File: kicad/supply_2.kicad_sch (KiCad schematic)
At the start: 24 parts, among them J2 +3.3, J3 GND, P1 USB_C_Plug_USB2.0, U3 TP4056-42-ESOP8, U4 USBLC6-2P6, U5 U8205A, U6 DW01A, U7 AMS1117-3.3, U8 Switch

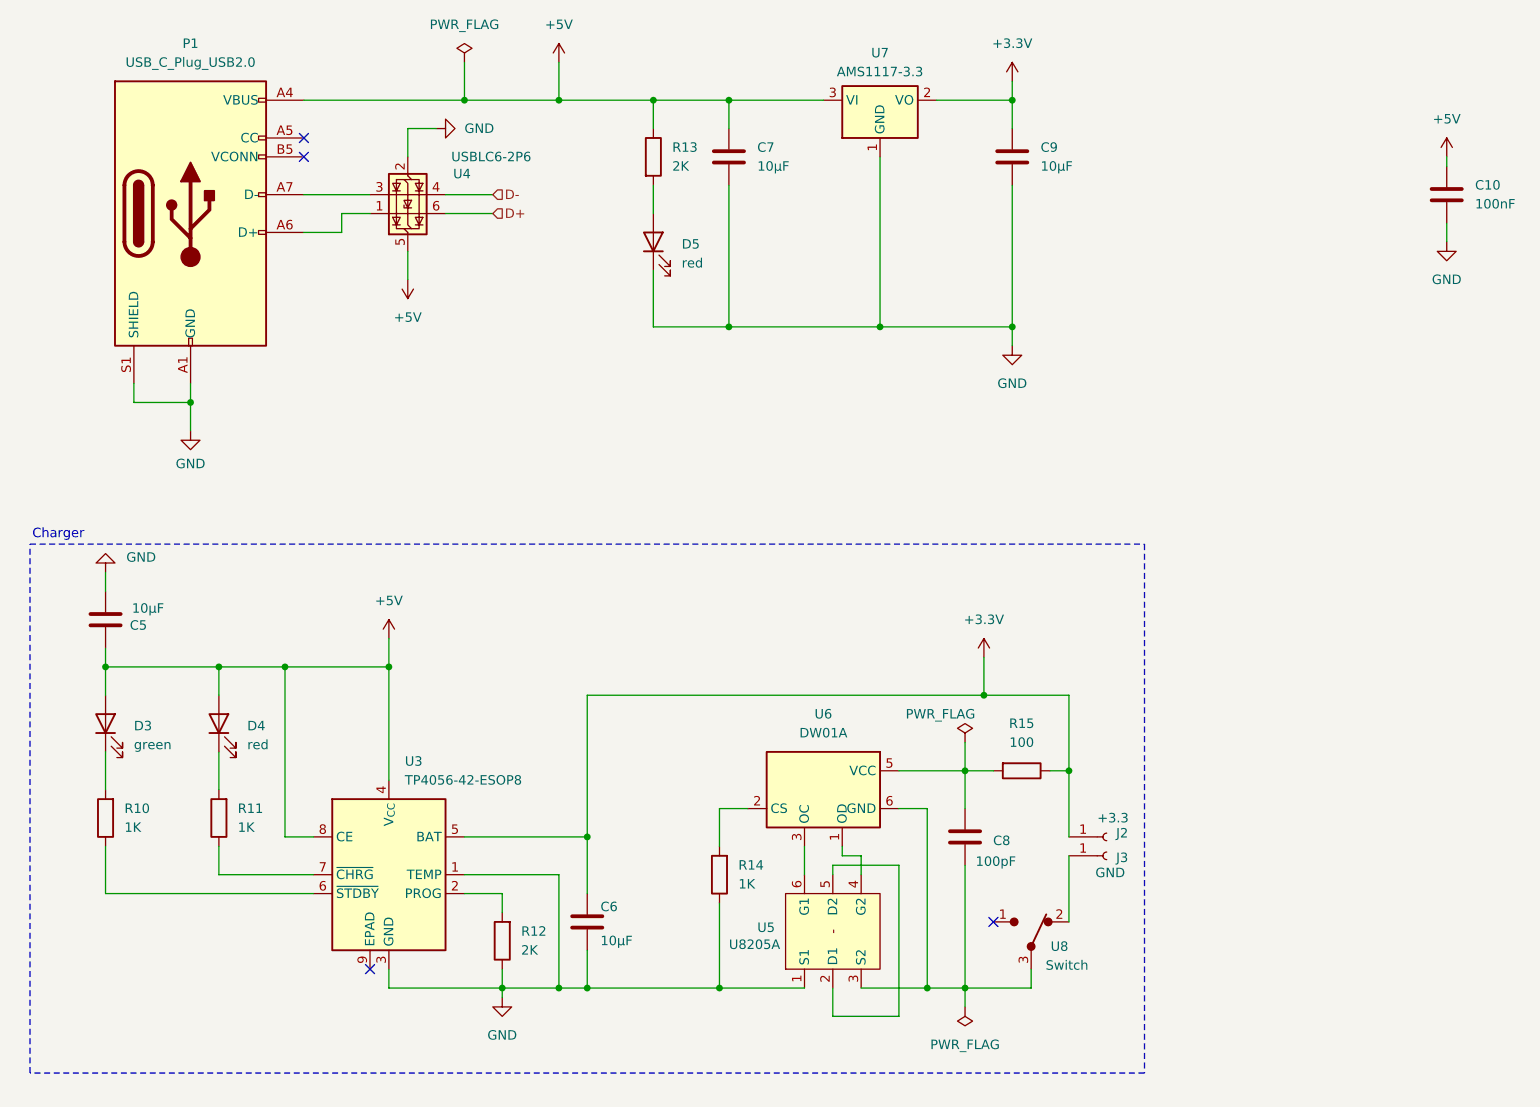
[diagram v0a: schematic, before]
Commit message: init
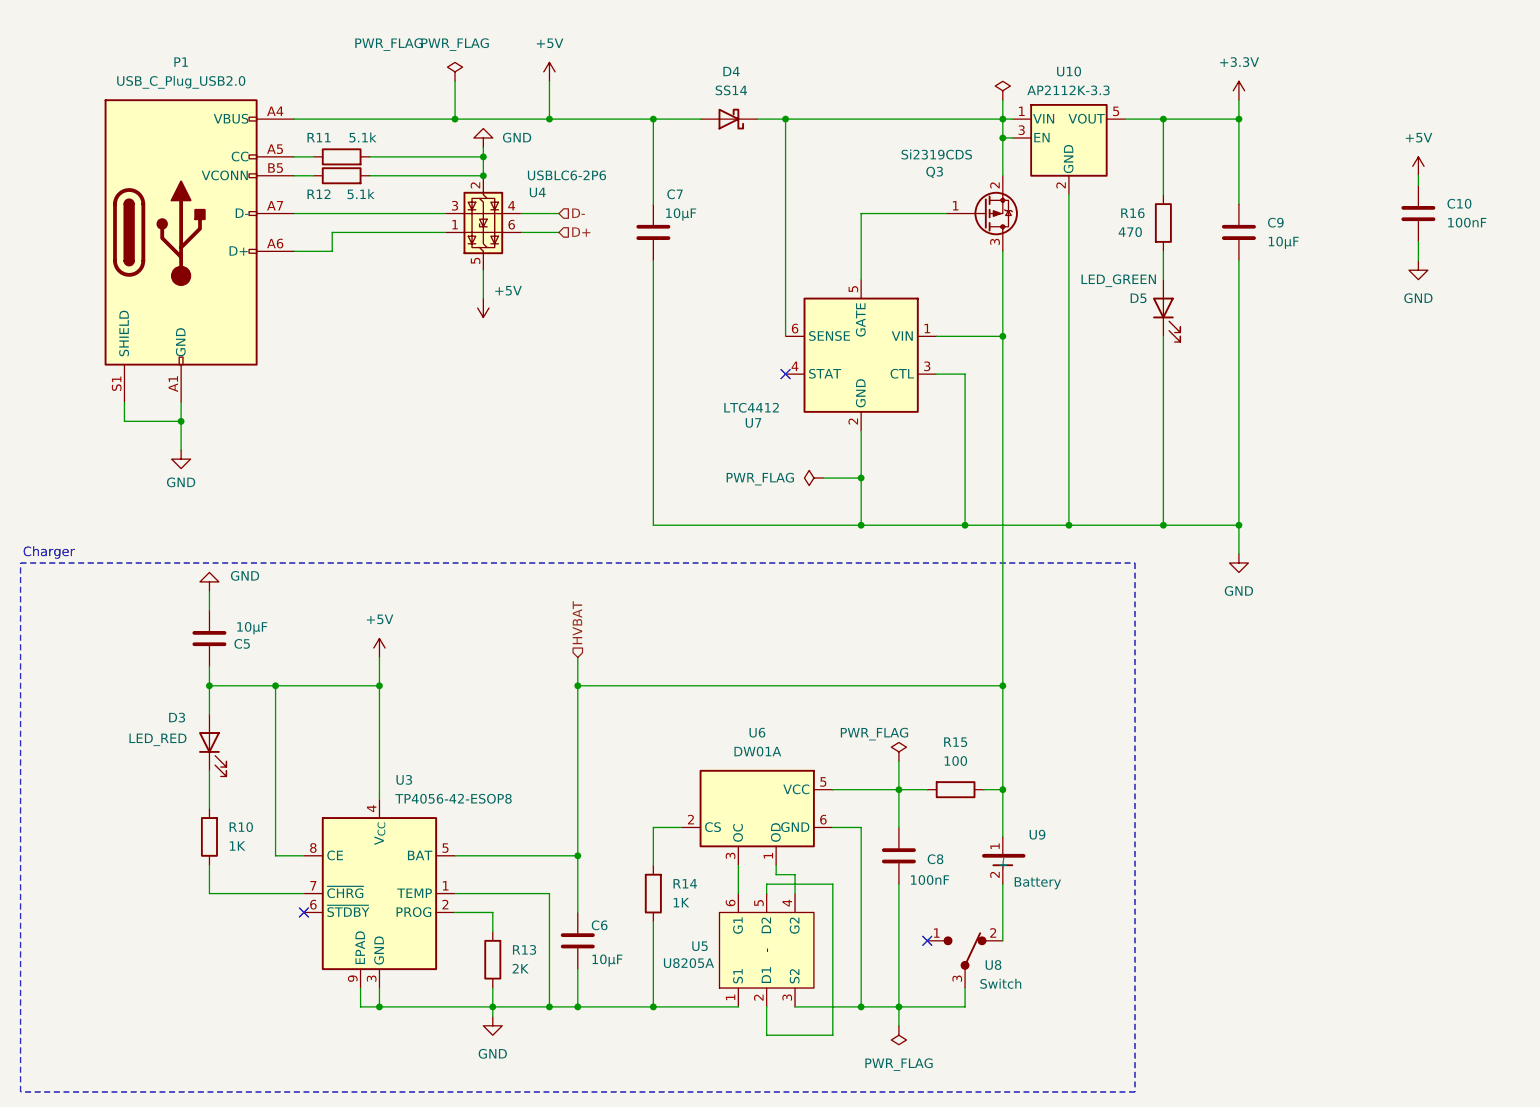
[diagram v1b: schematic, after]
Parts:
- removed D3: green, Diode_SMD:D_0603_1608Metric, symbol Device:LED
- removed J2: +3.3, TestPoint:TestPoint_THTPad_2.5x2.5mm_Drill1.2mm, symbol Connector:Conn_01x01_Socket
- removed J3: GND, TestPoint:TestPoint_THTPad_2.5x2.5mm_Drill1.2mm, symbol Connector:Conn_01x01_Socket
- removed U7: AMS1117-3.3, Package_TO_SOT_SMD:SOT-223-3_TabPin2, symbol Regulator_Linear:AMS1117-3.3
- added D4: SS14, Diode_SMD:D_SMA, symbol Diode:SS14
- added Q3: Si2319CDS, Package_TO_SOT_SMD:SOT-23, symbol Transistor_FET:Si2319CDS
- added R13: 2K, Resistor_SMD:R_0805_2012Metric, symbol Device:R
- added U10: AP2112K-3.3, Package_TO_SOT_SMD:SOT-23-5, symbol Regulator_Linear:AP2112K-3.3
- added U7: LTC4412, Package_TO_SOT_SMD:TSOT-23-6, symbol Power_Management:LTC4412xS6
- added U9: Battery, Battery:BatteryHolder_Keystone_1058_1x2032, symbol PCM_yvolodym:NCR18650B
- C10, C5, C6, C7, C9: footprint Capacitor_SMD:C_1206_3216Metric -> Capacitor_SMD:C_0805_2012Metric
- C8: value 100pF -> 100nF; footprint Capacitor_SMD:C_1206_3216Metric -> Capacitor_SMD:C_0805_2012Metric
- D3: renamed from D4; value red -> LED_RED; footprint Diode_SMD:D_0603_1608Metric -> Diode_SMD:D_0805_2012Metric
- D5: value red -> LED_GREEN; footprint Diode_SMD:D_0603_1608Metric -> Diode_SMD:D_0805_2012Metric
- R10, R14, R15: footprint Resistor_SMD:R_1206_3216Metric -> Resistor_SMD:R_0805_2012Metric
- R11: value 1K -> 5.1k; footprint Resistor_SMD:R_1206_3216Metric -> Resistor_SMD:R_0805_2012Metric
- R12: value 2K -> 5.1k; footprint Resistor_SMD:R_1206_3216Metric -> Resistor_SMD:R_0805_2012Metric
- R16: renamed from R13; value 2K -> 470; footprint Resistor_SMD:R_1206_3216Metric -> Resistor_SMD:R_0805_2012Metric
- U8: footprint PCM_yvolodym:Switch -> Button_Switch_SMD:SW_SPDT_PCM12
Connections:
- net +3.3V: now also R16.1, U10.5 (VOUT); no longer C6.1, R15.1, U3.5 (BAT)
- net +5V: now also D4.2 (A); no longer R16.1
- net GND: now also R11.2, R12.2, U3.9 (EPAD), R13.1, U10.2 (GND), U7.2 (GND), U7.3 (CTL); no longer R12.1
- net at D3.1 (K): now also R10.2; no longer R11.2
- net at U3.6 (~{STDBY}): no longer R10.1
- net at U8.2: now also U9.2 (-)
- net at P1.A5 (CC): now also R11.1
- net at P1.B5 (VCONN): now also R12.1
- net at U3.2 (PROG): now also R13.2; no longer R12.2
- net at U3.7 (~{CHRG}): now also R10.1; no longer R11.1
- new net: D4.1 (K), Q3.2 (S), U10.1 (VIN), U10.3 (EN), U7.6 (SENSE)
- new net: Q3.1 (G), U7.5 (GATE)
- new net HVBAT: C6.1, Q3.3 (D), R15.1, U3.5 (BAT), U7.1 (VIN), U9.1 (+)
- no-connect marks 4 -> 3
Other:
- moved on the sheet: C10, D3, D5, R14, R15, R16, U3, U4, U5, U6, U8

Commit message: init
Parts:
- U9: footprint Battery:BatteryHolder_Keystone_1058_1x2032 -> PCM_yvolodym:CR2032
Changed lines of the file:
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@@
 			)
 		)
-		(property "Footprint" "Battery:BatteryHolder_Keystone_1058_1x2032"
+		(property "Footprint" "PCM_yvolodym:CR2032"
 			(at 177.8 130.81 0)
 			(effects
@@
 			)
 		)
-		(property "Datasheet" "https://www.batteryspace.com/prod-specs/NCR18650B.pdf"
+		(property "Datasheet" ""
 			(at 177.8 130.81 0)
 			(effects
@@
 			)
 		)
-		(property "Description" "Panasonic NCR18650B 3.7V Li-ion 18650 cell"
+		(property "Description" "CR2032"
 			(at 177.8 130.81 0)
 			(effects
+				(font
+					(size 1.27 1.27)
+				)
+				(hide yes)
+			)
+		)
+		(property "LCSC" ""
+			(at 177.8 130.81 0)
+			(effects
